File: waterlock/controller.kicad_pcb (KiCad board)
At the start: 2 copper layers, 68.1 x 51.1 mm, 31 parts, among them CON1 AVR-ISP-10, J1 v5, J2 v12, J3 m1, J4 m2, J5 Battery, J6 L1, J7 L2, SW1 Turn, U1 ATMEGA8-16PU, U3 L293D

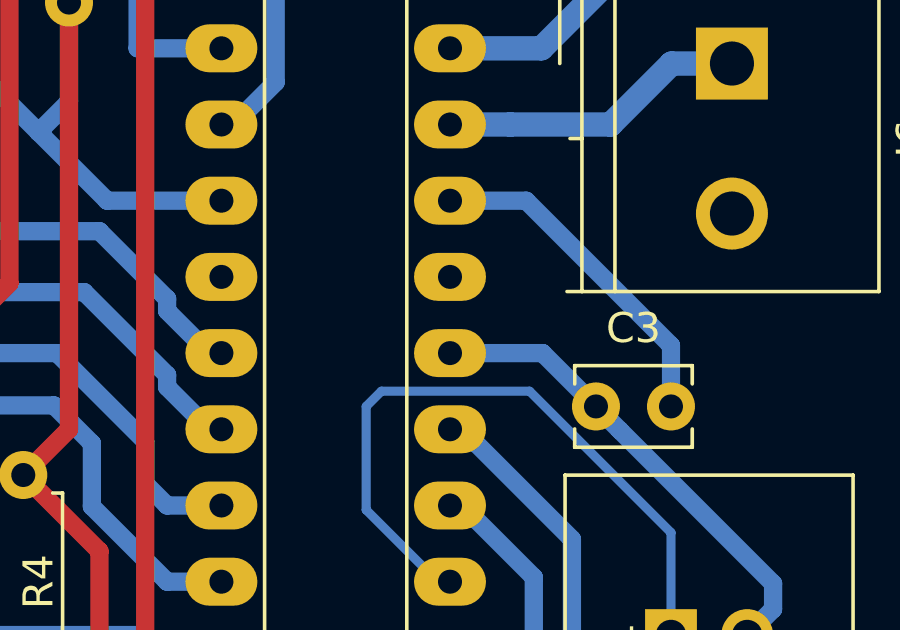
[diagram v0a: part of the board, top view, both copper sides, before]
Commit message: up01
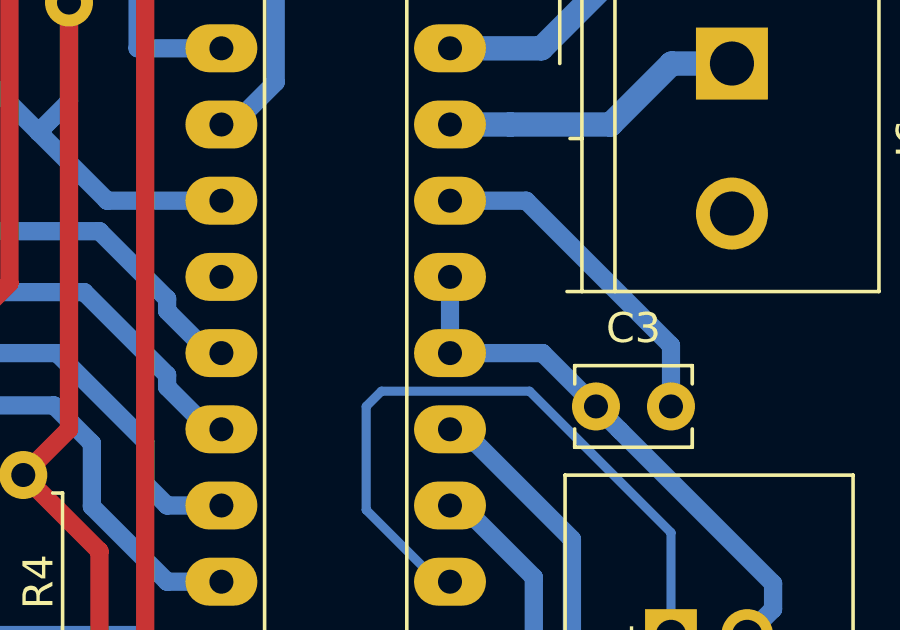
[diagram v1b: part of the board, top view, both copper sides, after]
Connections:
- U1 pad 21: Net-(U1-Pad21) -> +5V
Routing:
- net +5V: track 106.6 -> 110.2 mm
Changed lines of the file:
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@@
 (kicad_pcb (version 4) (host pcbnew 4.0.7-e2-6376~61~ubuntu18.04.1)
   (general
-    (links 71)
-    (no_connects 3)
+    (links 72)
+    (no_connects 2)
     (area 11.862999 12.116999 80.085001 63.321001)
     (thickness 1.6)
     (drawings 6)
-    (tracks 205)
+    (tracks 207)
     (zones 0)
     (modules 31)
-    (nets 37)
+    (nets 36)
   )
   (page A4)
@@
   (net 29 /m2a)
   (net 30 /en12)
-  (net 31 "Net-(U1-Pad21)")
-  (net 32 /m3a)
-  (net 33 /m4a)
-  (net 34 /en34)
-  (net 35 "Net-(U1-Pad27)")
-  (net 36 "Net-(U1-Pad28)")
+  (net 31 /m3a)
+  (net 32 /m4a)
+  (net 33 /en34)
+  (net 34 "Net-(U1-Pad27)")
+  (net 35 "Net-(U1-Pad28)")
   (net_class Default "This is the default net class."
     (clearance 0.2)
@@
     (add_net "Net-(U1-Pad16)")
     (add_net "Net-(U1-Pad2)")
-    (add_net "Net-(U1-Pad21)")
     (add_net "Net-(U1-Pad27)")
     (add_net "Net-(U1-Pad28)")
@@
       (net 6 +5V))
     (pad 21 thru_hole oval (at 7.62 17.78) (size 2.4 1.6) (drill 0.8) (layers *.Cu *.Mask)
-      (net 31 "Net-(U1-Pad21)"))
+      (net 6 +5V))
     (pad 8 thru_hole oval (at 0 17.78) (size 2.4 1.6) (drill 0.8) (layers *.Cu *.Mask)
       (net 2 GND))
@@
       (net 4 /Line2))
     (pad 11 thru_hole oval (at 0 25.4) (size 2.4 1.6) (drill 0.8) (layers *.Cu *.Mask)
-      (net 33 /m4a))
+      (net 32 /m4a))
     (pad 25 thru_hole oval (at 7.62 7.62) (size 2.4 1.6) (drill 0.8) (layers *.Cu *.Mask)
       (net 24 /pwr_c1))
     (pad 12 thru_hole oval (at 0 27.94) (size 2.4 1.6) (drill 0.8) (layers *.Cu *.Mask)
-      (net 32 /m3a))
+      (net 31 /m3a))
     (pad 26 thru_hole oval (at 7.62 5.08) (size 2.4 1.6) (drill 0.8) (layers *.Cu *.Mask)
       (net 22 /pwr_c2))
     (pad 13 thru_hole oval (at 0 30.48) (size 2.4 1.6) (drill 0.8) (layers *.Cu *.Mask)
-      (net 34 /en34))
+      (net 33 /en34))
     (pad 27 thru_hole oval (at 7.62 2.54) (size 2.4 1.6) (drill 0.8) (layers *.Cu *.Mask)
-      (net 35 "Net-(U1-Pad27)"))
+      (net 34 "Net-(U1-Pad27)"))
     (pad 14 thru_hole oval (at 0 33.02) (size 2.4 1.6) (drill 0.8) (layers *.Cu *.Mask)
       (net 23 /btn_1))
     (pad 28 thru_hole oval (at 7.62 0) (size 2.4 1.6) (drill 0.8) (layers *.Cu *.Mask)
-      (net 36 "Net-(U1-Pad28)"))
+      (net 35 "Net-(U1-Pad28)"))
     (model ${KISYS3DMOD}/Housings_DIP.3dshapes/DIP-28_W7.62mm_LongPads.wrl
       (at (xyz 0 0 0))
@@
       (net 30 /en12))
     (pad 9 thru_hole oval (at 7.62 17.78 270) (size 1.6 1.6) (drill 0.8) (layers *.Cu *.Mask)
-      (net 34 /en34))
+      (net 33 /en34))
     (pad 2 thru_hole oval (at 0 2.54 270) (size 1.6 1.6) (drill 0.8) (layers *.Cu *.Mask)
       (net 28 /m1a))
     (pad 10 thru_hole oval (at 7.62 15.24 270) (size 1.6 1.6) (drill 0.8) (layers *.Cu *.Mask)
-      (net 32 /m3a))
+      (net 31 /m3a))
     (pad 3 thru_hole oval (at 0 5.08 270) (size 1.6 1.6) (drill 0.8) (layers *.Cu *.Mask)
       (net 18 "Net-(J3-Pad1)"))
@@
       (net 29 /m2a))
     (pad 15 thru_hole oval (at 7.62 2.54 270) (size 1.6 1.6) (drill 0.8) (layers *.Cu *.Mask)
-      (net 33 /m4a))
+      (net 32 /m4a))
     (pad 8 thru_hole oval (at 0 17.78 270) (size 1.6 1.6) (drill 0.8) (layers *.Cu *.Mask)
       (net 11 +12V))
@@
   (segment (start 61.214 43.58) (end 63.608 45.974) (width 0.3048) (layer B.Cu) (net 5))
   (segment (start 63.608 45.974) (end 64.008 45.974) (width 0.3048) (layer B.Cu) (net 5))
+  (segment (start 64.008 35.814) (end 64.008 38.354) (width 0.6096) (layer B.Cu) (net 6))
+  (segment (start 64.008 35.814) (end 64.008 36.864) (width 0.25) (layer B.Cu) (net 6))
   (segment (start 49.784 42.418) (end 52.324 44.958) (width 0.6096) (layer F.Cu) (net 6))
   (segment (start 52.324 44.958) (end 52.324 56.607199) (width 0.6096) (layer F.Cu) (net 6))
@@
   (segment (start 58.1976 29.3244) (end 56.788 30.734) (width 0.6096) (layer B.Cu) (net 30))
   (segment (start 56.788 30.734) (end 56.388 30.734) (width 0.6096) (layer B.Cu) (net 30))
-  (segment (start 50.80592 40.097199) (end 52.07 41.361279) (width 0.6096) (layer B.Cu) (net 32))
-  (segment (start 56.388 45.974) (end 54.5784 45.974) (width 0.6096) (layer B.Cu) (net 32))
-  (segment (start 54.5784 45.974) (end 52.07 43.4656) (width 0.6096) (layer B.Cu) (net 32))
-  (segment (start 52.07 43.4656) (end 52.07 41.361279) (width 0.6096) (layer B.Cu) (net 32))
-  (segment (start 30.226 26.162) (end 35.477589 31.413589) (width 0.6096) (layer B.Cu) (net 32))
-  (segment (start 35.477589 31.413589) (end 35.477589 36.775656) (width 0.6096) (layer B.Cu) (net 32))
-  (segment (start 35.477589 36.775656) (end 38.799132 40.097199) (width 0.6096) (layer B.Cu) (net 32))
-  (segment (start 38.799132 40.097199) (end 50.80592 40.097199) (width 0.6096) (layer B.Cu) (net 32))
-  (segment (start 50.908 38.354) (end 53.848 41.294) (width 0.6096) (layer B.Cu) (net 33))
-  (segment (start 56.388 43.434) (end 54.5784 43.434) (width 0.6096) (layer B.Cu) (net 33))
-  (segment (start 54.5784 43.434) (end 53.848 42.7036) (width 0.6096) (layer B.Cu) (net 33))
-  (segment (start 53.848 42.7036) (end 53.848 41.294) (width 0.6096) (layer B.Cu) (net 33))
-  (segment (start 38.200894 38.354) (end 50.908 38.354) (width 0.6096) (layer B.Cu) (net 33))
-  (segment (start 42.926 26.162) (end 41.621199 27.466801) (width 0.6096) (layer B.Cu) (net 33))
-  (segment (start 36.287199 31.123695) (end 36.287199 36.440305) (width 0.6096) (layer B.Cu) (net 33))
-  (segment (start 41.621199 27.466801) (end 39.944093 27.466801) (width 0.6096) (layer B.Cu) (net 33))
-  (segment (start 39.944093 27.466801) (end 36.287199 31.123695) (width 0.6096) (layer B.Cu) (net 33))
-  (segment (start 36.287199 36.440305) (end 38.200894 38.354) (width 0.6096) (layer B.Cu) (net 33))
-  (segment (start 56.388 48.514) (end 54.5784 48.514) (width 0.6096) (layer B.Cu) (net 34))
-  (segment (start 53.8164 47.752) (end 42.264894 47.752) (width 0.6096) (layer B.Cu) (net 34))
-  (segment (start 54.5784 48.514) (end 53.8164 47.752) (width 0.6096) (layer B.Cu) (net 34))
-  (segment (start 42.264894 47.752) (end 40.386 45.873106) (width 0.6096) (layer B.Cu) (net 34))
-  (segment (start 40.386 45.873106) (end 40.386 43.942) (width 0.6096) (layer B.Cu) (net 34))
-  (segment (start 40.386 43.942) (end 34.29 37.846) (width 0.6096) (layer B.Cu) (net 34))
-  (segment (start 34.29 37.846) (end 34.29 32.766) (width 0.6096) (layer B.Cu) (net 34))
-  (segment (start 34.29 32.766) (end 27.686 26.162) (width 0.6096) (layer B.Cu) (net 34))
+  (segment (start 50.80592 40.097199) (end 52.07 41.361279) (width 0.6096) (layer B.Cu) (net 31))
+  (segment (start 56.388 45.974) (end 54.5784 45.974) (width 0.6096) (layer B.Cu) (net 31))
+  (segment (start 54.5784 45.974) (end 52.07 43.4656) (width 0.6096) (layer B.Cu) (net 31))
+  (segment (start 52.07 43.4656) (end 52.07 41.361279) (width 0.6096) (layer B.Cu) (net 31))
+  (segment (start 30.226 26.162) (end 35.477589 31.413589) (width 0.6096) (layer B.Cu) (net 31))
+  (segment (start 35.477589 31.413589) (end 35.477589 36.775656) (width 0.6096) (layer B.Cu) (net 31))
+  (segment (start 35.477589 36.775656) (end 38.799132 40.097199) (width 0.6096) (layer B.Cu) (net 31))
+  (segment (start 38.799132 40.097199) (end 50.80592 40.097199) (width 0.6096) (layer B.Cu) (net 31))
+  (segment (start 50.908 38.354) (end 53.848 41.294) (width 0.6096) (layer B.Cu) (net 32))
+  (segment (start 56.388 43.434) (end 54.5784 43.434) (width 0.6096) (layer B.Cu) (net 32))
+  (segment (start 54.5784 43.434) (end 53.848 42.7036) (width 0.6096) (layer B.Cu) (net 32))
+  (segment (start 53.848 42.7036) (end 53.848 41.294) (width 0.6096) (layer B.Cu) (net 32))
+  (segment (start 38.200894 38.354) (end 50.908 38.354) (width 0.6096) (layer B.Cu) (net 32))
+  (segment (start 42.926 26.162) (end 41.621199 27.466801) (width 0.6096) (layer B.Cu) (net 32))
+  (segment (start 36.287199 31.123695) (end 36.287199 36.440305) (width 0.6096) (layer B.Cu) (net 32))
+  (segment (start 41.621199 27.466801) (end 39.944093 27.466801) (width 0.6096) (layer B.Cu) (net 32))
+  (segment (start 39.944093 27.466801) (end 36.287199 31.123695) (width 0.6096) (layer B.Cu) (net 32))
+  (segment (start 36.287199 36.440305) (end 38.200894 38.354) (width 0.6096) (layer B.Cu) (net 32))
+  (segment (start 56.388 48.514) (end 54.5784 48.514) (width 0.6096) (layer B.Cu) (net 33))
+  (segment (start 53.8164 47.752) (end 42.264894 47.752) (width 0.6096) (layer B.Cu) (net 33))
+  (segment (start 54.5784 48.514) (end 53.8164 47.752) (width 0.6096) (layer B.Cu) (net 33))
+  (segment (start 42.264894 47.752) (end 40.386 45.873106) (width 0.6096) (layer B.Cu) (net 33))
+  (segment (start 40.386 45.873106) (end 40.386 43.942) (width 0.6096) (layer B.Cu) (net 33))
+  (segment (start 40.386 43.942) (end 34.29 37.846) (width 0.6096) (layer B.Cu) (net 33))
+  (segment (start 34.29 37.846) (end 34.29 32.766) (width 0.6096) (layer B.Cu) (net 33))
+  (segment (start 34.29 32.766) (end 27.686 26.162) (width 0.6096) (layer B.Cu) (net 33))
   (zone (net 2) (net_name GND) (layer B.Cu) (hatch edge 0.508)
     (connect_pads (clearance 0.508))
